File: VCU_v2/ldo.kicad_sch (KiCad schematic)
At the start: 8 parts, among them U1 XC6221B481MR-G, U3 AMS1117-3.3

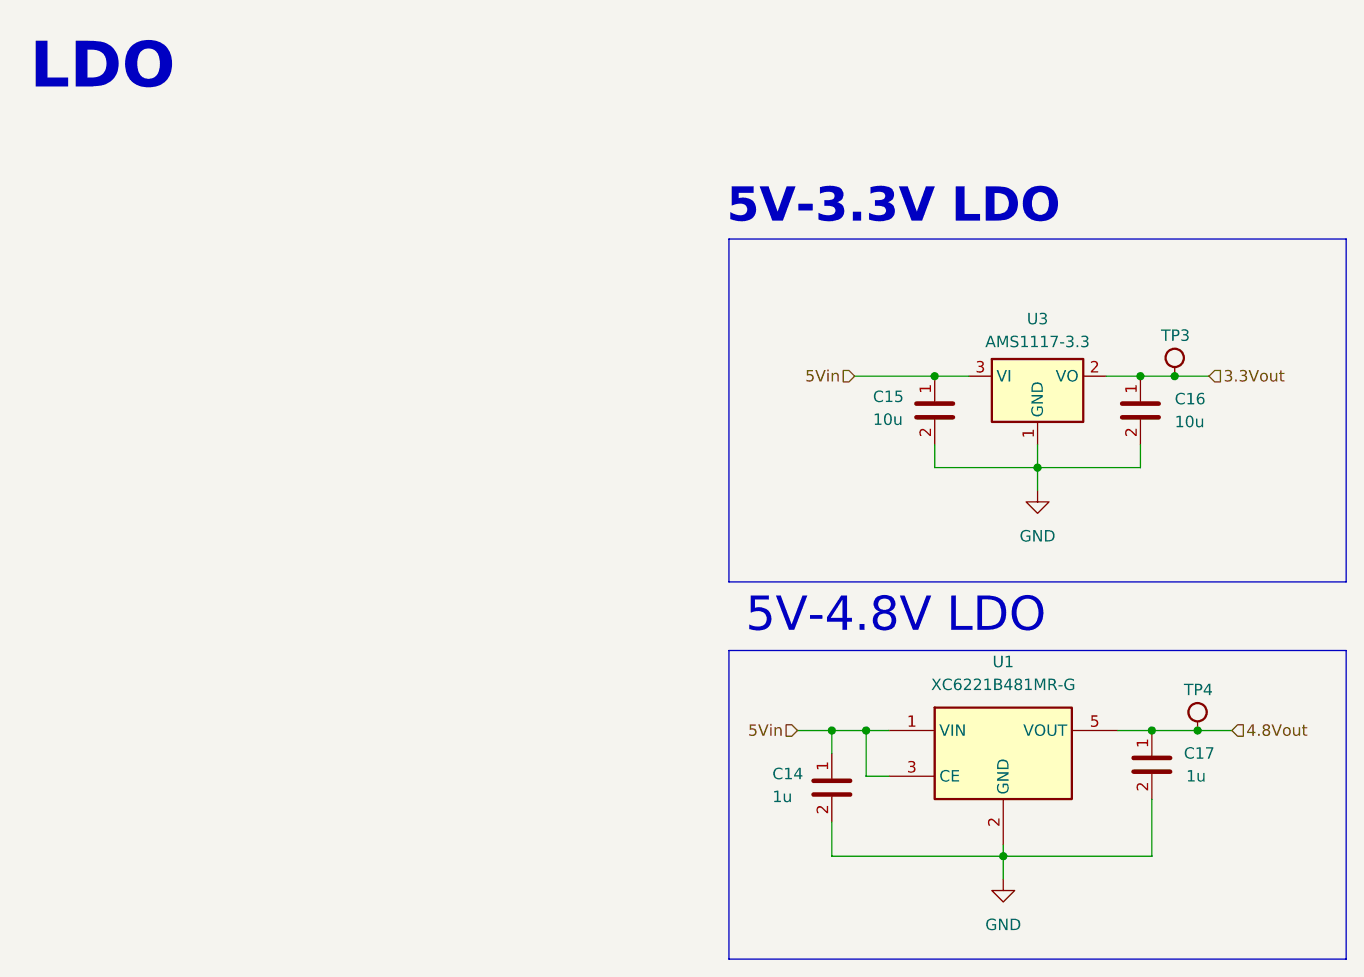
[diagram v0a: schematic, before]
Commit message: vcu v2 schematics done
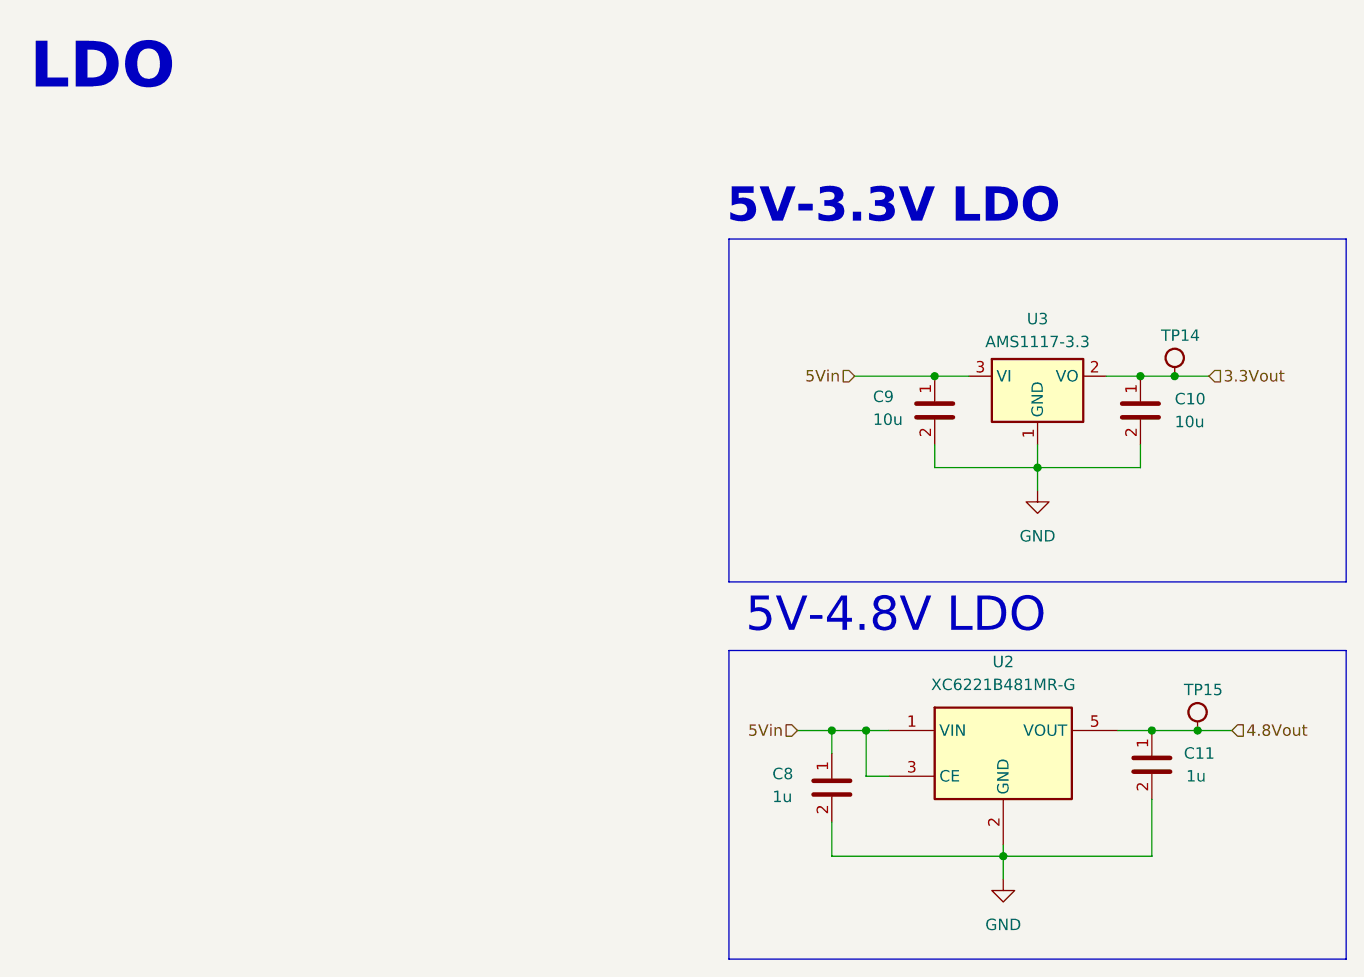
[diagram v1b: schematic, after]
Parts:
- renumbered C16 to C10, C17 to C11, C14 to C8, C15 to C9, TP3 to TP14, TP4 to TP15, U1 to U2
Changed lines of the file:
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@@
 		(dnp no)
 		(fields_autoplaced yes)
-		(property "Reference" "#PWR032"
+		(property "Reference" "#PWR023"
 			(at 121.92 115.57 0)
 			(effects
@@
 			(project ""
 				(path "/4ee6c2ad-9a1b-4276-b3cf-1cc8dc52967e/9e4b5f8d-93dc-46d5-aa92-d0e0d2e07b3d/672d0e35-df5b-43af-b77f-286811b03e69"
-					(reference "#PWR032")
+					(reference "#PWR023")
 					(unit 1)
 				)
@@
 		(on_board yes)
 		(dnp no)
-		(property "Reference" "C17"
+		(property "Reference" "C11"
 			(at 141.986 95.25 0)
 			(effects
@@
 			(project ""
 				(path "/4ee6c2ad-9a1b-4276-b3cf-1cc8dc52967e/9e4b5f8d-93dc-46d5-aa92-d0e0d2e07b3d/672d0e35-df5b-43af-b77f-286811b03e69"
-					(reference "C17")
+					(reference "C11")
 					(unit 1)
 				)
@@
 		(on_board yes)
 		(dnp no)
-		(property "Reference" "C15"
+		(property "Reference" "C9"
 			(at 107.442 55.626 0)
 			(effects
@@
 			(project ""
 				(path "/4ee6c2ad-9a1b-4276-b3cf-1cc8dc52967e/9e4b5f8d-93dc-46d5-aa92-d0e0d2e07b3d/672d0e35-df5b-43af-b77f-286811b03e69"
-					(reference "C15")
+					(reference "C9")
 					(unit 1)
 				)
@@
 		(dnp no)
 		(fields_autoplaced yes)
-		(property "Reference" "C16"
+		(property "Reference" "C10"
 			(at 140.97 55.8799 0)
 			(effects
@@
 			(project ""
 				(path "/4ee6c2ad-9a1b-4276-b3cf-1cc8dc52967e/9e4b5f8d-93dc-46d5-aa92-d0e0d2e07b3d/672d0e35-df5b-43af-b77f-286811b03e69"
-					(reference "C16")
+					(reference "C10")
 					(unit 1)
 				)
@@
 		(dnp no)
 		(fields_autoplaced yes)
-		(property "Reference" "U1"
+		(property "Reference" "U2"
 			(at 121.92 85.09 0)
 			(effects
@@
 			(project ""
 				(path "/4ee6c2ad-9a1b-4276-b3cf-1cc8dc52967e/9e4b5f8d-93dc-46d5-aa92-d0e0d2e07b3d/672d0e35-df5b-43af-b77f-286811b03e69"
-					(reference "U1")
+					(reference "U2")
 					(unit 1)
 				)
@@
 		(on_board yes)
 		(dnp no)
-		(property "Reference" "TP3"
+		(property "Reference" "TP14"
 			(at 139.4468 48.0837 0)
 			(effects
@@
 			(project "VCU_v1"
 				(path "/4ee6c2ad-9a1b-4276-b3cf-1cc8dc52967e/9e4b5f8d-93dc-46d5-aa92-d0e0d2e07b3d/672d0e35-df5b-43af-b77f-286811b03e69"
-					(reference "TP3")
+					(reference "TP14")
 					(unit 1)
 				)
@@
 		(dnp no)
 		(fields_autoplaced yes)
-		(property "Reference" "#PWR031"
+		(property "Reference" "#PWR024"
 			(at 125.73 72.39 0)
 			(effects
@@
 			(project ""
 				(path "/4ee6c2ad-9a1b-4276-b3cf-1cc8dc52967e/9e4b5f8d-93dc-46d5-aa92-d0e0d2e07b3d/672d0e35-df5b-43af-b77f-286811b03e69"
-					(reference "#PWR031")
+					(reference "#PWR024")
 					(unit 1)
 				)
@@
 		(on_board yes)
 		(dnp no)
-		(property "Reference" "TP4"
+		(property "Reference" "TP15"
 			(at 141.9868 87.4537 0)
 			(effects
@@
 			(project "VCU_v1"
 				(path "/4ee6c2ad-9a1b-4276-b3cf-1cc8dc52967e/9e4b5f8d-93dc-46d5-aa92-d0e0d2e07b3d/672d0e35-df5b-43af-b77f-286811b03e69"
-					(reference "TP4")
+					(reference "TP15")
 					(unit 1)
 				)
@@
 		(on_board yes)
 		(dnp no)
-		(property "Reference" "C14"
+		(property "Reference" "C8"
 			(at 96.266 97.536 0)
 			(effects
@@
 			(project ""
 				(path "/4ee6c2ad-9a1b-4276-b3cf-1cc8dc52967e/9e4b5f8d-93dc-46d5-aa92-d0e0d2e07b3d/672d0e35-df5b-43af-b77f-286811b03e69"
-					(reference "C14")
+					(reference "C8")
 					(unit 1)
 				)

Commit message: placements friggin 80% friggin done shoutout epstein
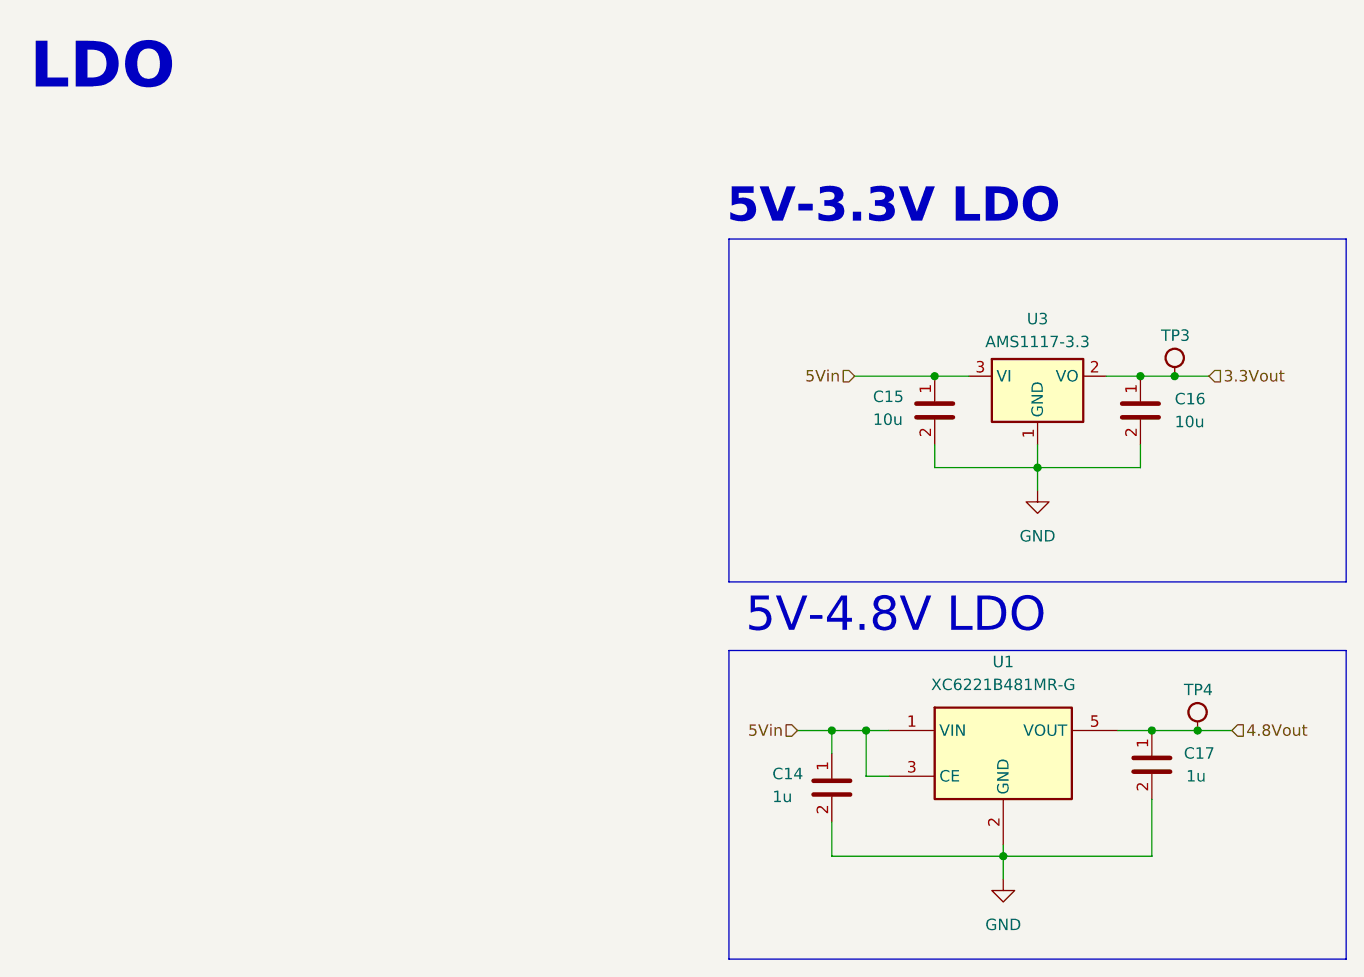
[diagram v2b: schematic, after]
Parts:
- renumbered C8 to C14, C9 to C15, C10 to C16, C11 to C17, TP14 to TP3, TP15 to TP4, U2 to U1
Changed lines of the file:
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@@
 		(dnp no)
 		(fields_autoplaced yes)
-		(property "Reference" "#PWR023"
+		(property "Reference" "#PWR032"
 			(at 121.92 115.57 0)
 			(effects
@@
 			(project ""
 				(path "/4ee6c2ad-9a1b-4276-b3cf-1cc8dc52967e/9e4b5f8d-93dc-46d5-aa92-d0e0d2e07b3d/672d0e35-df5b-43af-b77f-286811b03e69"
-					(reference "#PWR023")
+					(reference "#PWR032")
 					(unit 1)
 				)
@@
 		(on_board yes)
 		(dnp no)
-		(property "Reference" "C11"
+		(property "Reference" "C17"
 			(at 141.986 95.25 0)
 			(effects
@@
 			(project ""
 				(path "/4ee6c2ad-9a1b-4276-b3cf-1cc8dc52967e/9e4b5f8d-93dc-46d5-aa92-d0e0d2e07b3d/672d0e35-df5b-43af-b77f-286811b03e69"
-					(reference "C11")
+					(reference "C17")
 					(unit 1)
 				)
@@
 		(on_board yes)
 		(dnp no)
-		(property "Reference" "C9"
+		(property "Reference" "C15"
 			(at 107.442 55.626 0)
 			(effects
@@
 			(project ""
 				(path "/4ee6c2ad-9a1b-4276-b3cf-1cc8dc52967e/9e4b5f8d-93dc-46d5-aa92-d0e0d2e07b3d/672d0e35-df5b-43af-b77f-286811b03e69"
-					(reference "C9")
+					(reference "C15")
 					(unit 1)
 				)
@@
 		(dnp no)
 		(fields_autoplaced yes)
-		(property "Reference" "C10"
+		(property "Reference" "C16"
 			(at 140.97 55.8799 0)
 			(effects
@@
 			(project ""
 				(path "/4ee6c2ad-9a1b-4276-b3cf-1cc8dc52967e/9e4b5f8d-93dc-46d5-aa92-d0e0d2e07b3d/672d0e35-df5b-43af-b77f-286811b03e69"
-					(reference "C10")
+					(reference "C16")
 					(unit 1)
 				)
@@
 		(dnp no)
 		(fields_autoplaced yes)
-		(property "Reference" "U2"
+		(property "Reference" "U1"
 			(at 121.92 85.09 0)
 			(effects
@@
 			(project ""
 				(path "/4ee6c2ad-9a1b-4276-b3cf-1cc8dc52967e/9e4b5f8d-93dc-46d5-aa92-d0e0d2e07b3d/672d0e35-df5b-43af-b77f-286811b03e69"
-					(reference "U2")
+					(reference "U1")
 					(unit 1)
 				)
@@
 		(on_board yes)
 		(dnp no)
-		(property "Reference" "TP14"
+		(property "Reference" "TP3"
 			(at 139.4468 48.0837 0)
 			(effects
@@
 			(project "VCU_v1"
 				(path "/4ee6c2ad-9a1b-4276-b3cf-1cc8dc52967e/9e4b5f8d-93dc-46d5-aa92-d0e0d2e07b3d/672d0e35-df5b-43af-b77f-286811b03e69"
-					(reference "TP14")
+					(reference "TP3")
 					(unit 1)
 				)
@@
 		(dnp no)
 		(fields_autoplaced yes)
-		(property "Reference" "#PWR024"
+		(property "Reference" "#PWR031"
 			(at 125.73 72.39 0)
 			(effects
@@
 			(project ""
 				(path "/4ee6c2ad-9a1b-4276-b3cf-1cc8dc52967e/9e4b5f8d-93dc-46d5-aa92-d0e0d2e07b3d/672d0e35-df5b-43af-b77f-286811b03e69"
-					(reference "#PWR024")
+					(reference "#PWR031")
 					(unit 1)
 				)
@@
 		(on_board yes)
 		(dnp no)
-		(property "Reference" "TP15"
+		(property "Reference" "TP4"
 			(at 141.9868 87.4537 0)
 			(effects
@@
 			(project "VCU_v1"
 				(path "/4ee6c2ad-9a1b-4276-b3cf-1cc8dc52967e/9e4b5f8d-93dc-46d5-aa92-d0e0d2e07b3d/672d0e35-df5b-43af-b77f-286811b03e69"
-					(reference "TP15")
+					(reference "TP4")
 					(unit 1)
 				)
@@
 		(on_board yes)
 		(dnp no)
-		(property "Reference" "C8"
+		(property "Reference" "C14"
 			(at 96.266 97.536 0)
 			(effects
@@
 			(project ""
 				(path "/4ee6c2ad-9a1b-4276-b3cf-1cc8dc52967e/9e4b5f8d-93dc-46d5-aa92-d0e0d2e07b3d/672d0e35-df5b-43af-b77f-286811b03e69"
-					(reference "C8")
+					(reference "C14")
 					(unit 1)
 				)
